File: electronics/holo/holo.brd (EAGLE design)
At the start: 164.8 x 150.7 mm, 63 parts, among them IC1 FT232L, U1 MT3608, U2 ESP32-WROOM-32E_(16MB), U3 IRLMS2002TRPBF, U4 IRLMS2002TRPBF

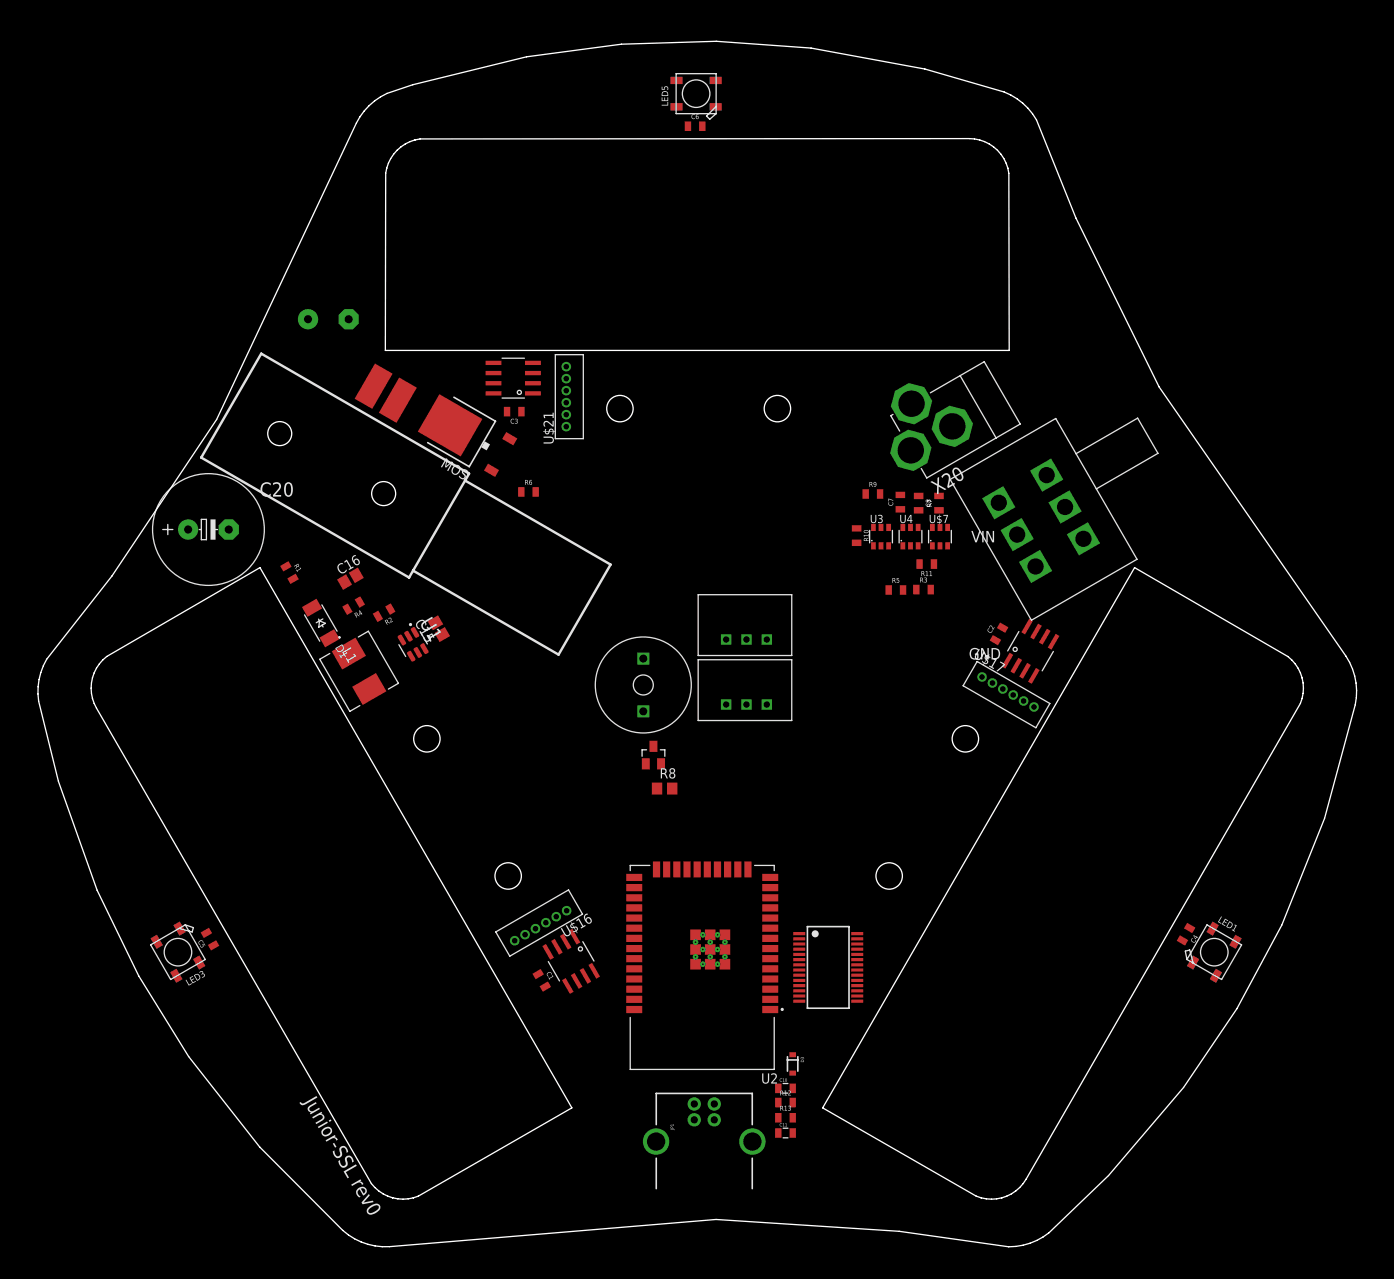
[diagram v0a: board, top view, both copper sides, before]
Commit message: Rework done
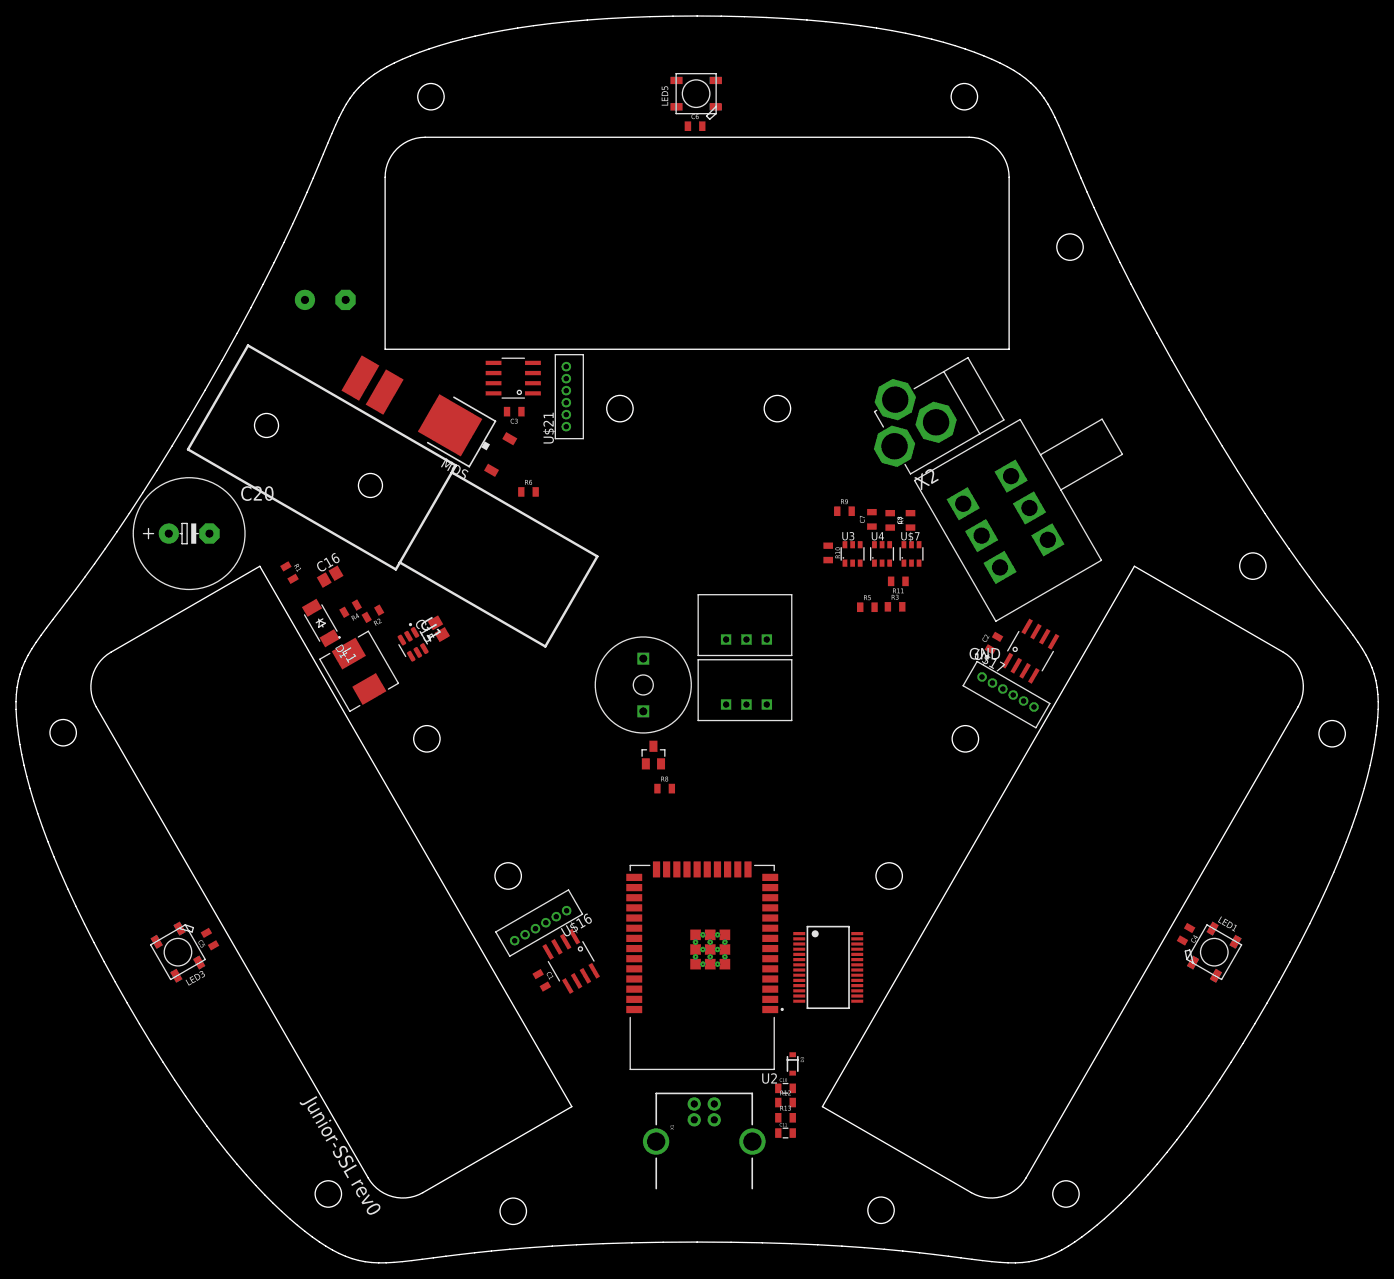
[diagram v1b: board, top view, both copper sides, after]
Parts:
- removed U$1: KICKER, rhoban:KICKER
- removed X20: (no value), powersupply:DC-21MM
- added KICK_PADS: KICKER, rhoban:KICKER
- added U$10, U$11, U$15, U$2, U$3, U$4, U$5, U$6, U$8, U$9: (no value), SparkFun-Electromechanical:STAND-OFF
- added X2: (no value), powersupply:DC-21MM
- R8: device rcl:R0805 -> SparkFun-Resistors:0805
- moved U$14 4.45 mm to (35.7, 17.1)
- moved R11 4.16 mm to (25.3, 11.4)
- moved R5 4.16 mm to (21.4, 8.19)
- moved U$7 4.16 mm to (26.9, 14.9)
- moved U3 4.16 mm to (19.6, 14.9)
- moved U4 4.16 mm to (23.2, 14.9)
- moved C7 4.16 mm to (22.0, 19.2)
- moved R7 4.16 mm to (26.8, 19.1)
- moved R3 4.16 mm to (24.9, 8.24)
- moved C8 4.16 mm to (24.3, 19.1)
- moved R10 4.16 mm to (16.5, 15.0)
- moved R9 4.16 mm to (18.5, 20.2)
- moved C16 2.55 mm to (-45.7, 12.0)
- moved C20 2.47 mm to (-63.4, 17.4)
- moved C19 2.44 mm to (-46.4, 46.6)
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- renumbered JP1 to X1
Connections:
- net 1: now also X2.1; no longer X20.1
- net GND_RAW: now also X2.3; no longer X20.3
- net KICKER: now also KICK_PADS.2; no longer U$1.2
- net N$7: now also X2.2; no longer X20.2
- net VSTORE: now also KICK_PADS.1; no longer U$1.1
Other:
- board size 164.8 x 150.7 mm -> 170.3 x 155.9 mm
- board text removed: "VIN"
